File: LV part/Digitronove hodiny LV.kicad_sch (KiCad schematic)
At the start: 92 parts, among them J1 DD4012SB_3V3, J10 Output, J11 Output, J12 Output, J13 -, J14 9V to 170V, J15 Output, J16 Output, J17 Output, J18 Output, J19 Output, J2 +, J20 Output, J21 Output, J22 Output, J24 RCWL-0516, J25 Output, J26 Output, J27 Output, J28 Output, J29 Output, J3 Output, J30 Output, J31 Output, J32 Output, J33 Output, J34 Output, J35 Output, J36 Output, J37 Output, J38 Output, J39 Output, J4 Output, J40 Output, J41 Output, J42 Output, J43 Output, J5 Output, J6 Output, J7 Output, J8 Output, J9 Output, SW1 RESET, SW2 START/STOP, SW3 +1, SW4 SWITCH, U1 74HC595, U2 74HC595, U3 ESP32-WROOM-32, U4 74HC595, U5 74HC595, U6 74HC595, U7 74HC595

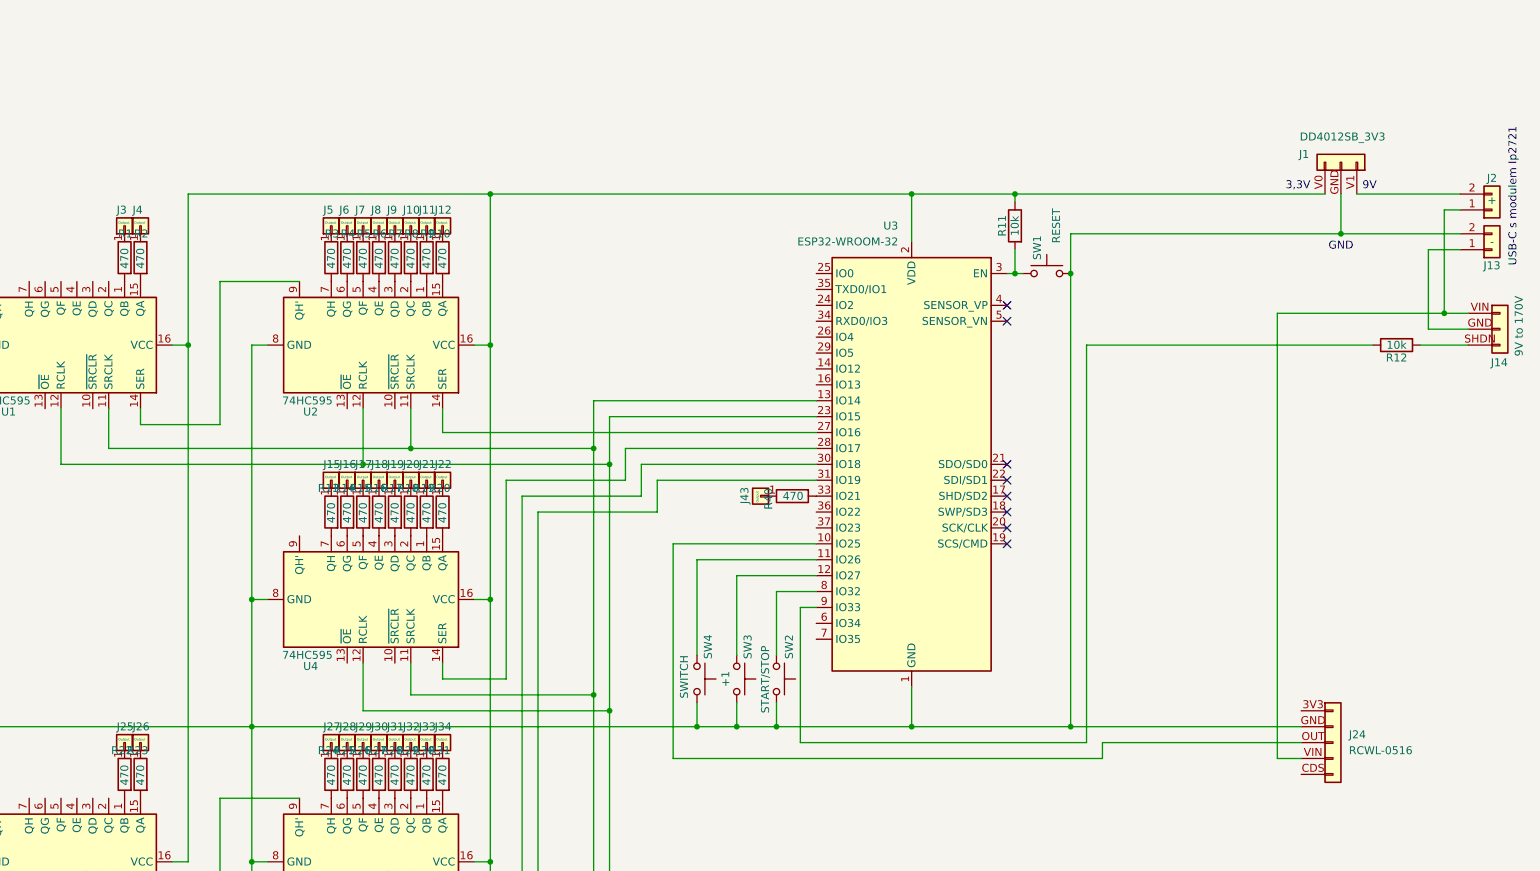
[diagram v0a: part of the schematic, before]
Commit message: LV Schema
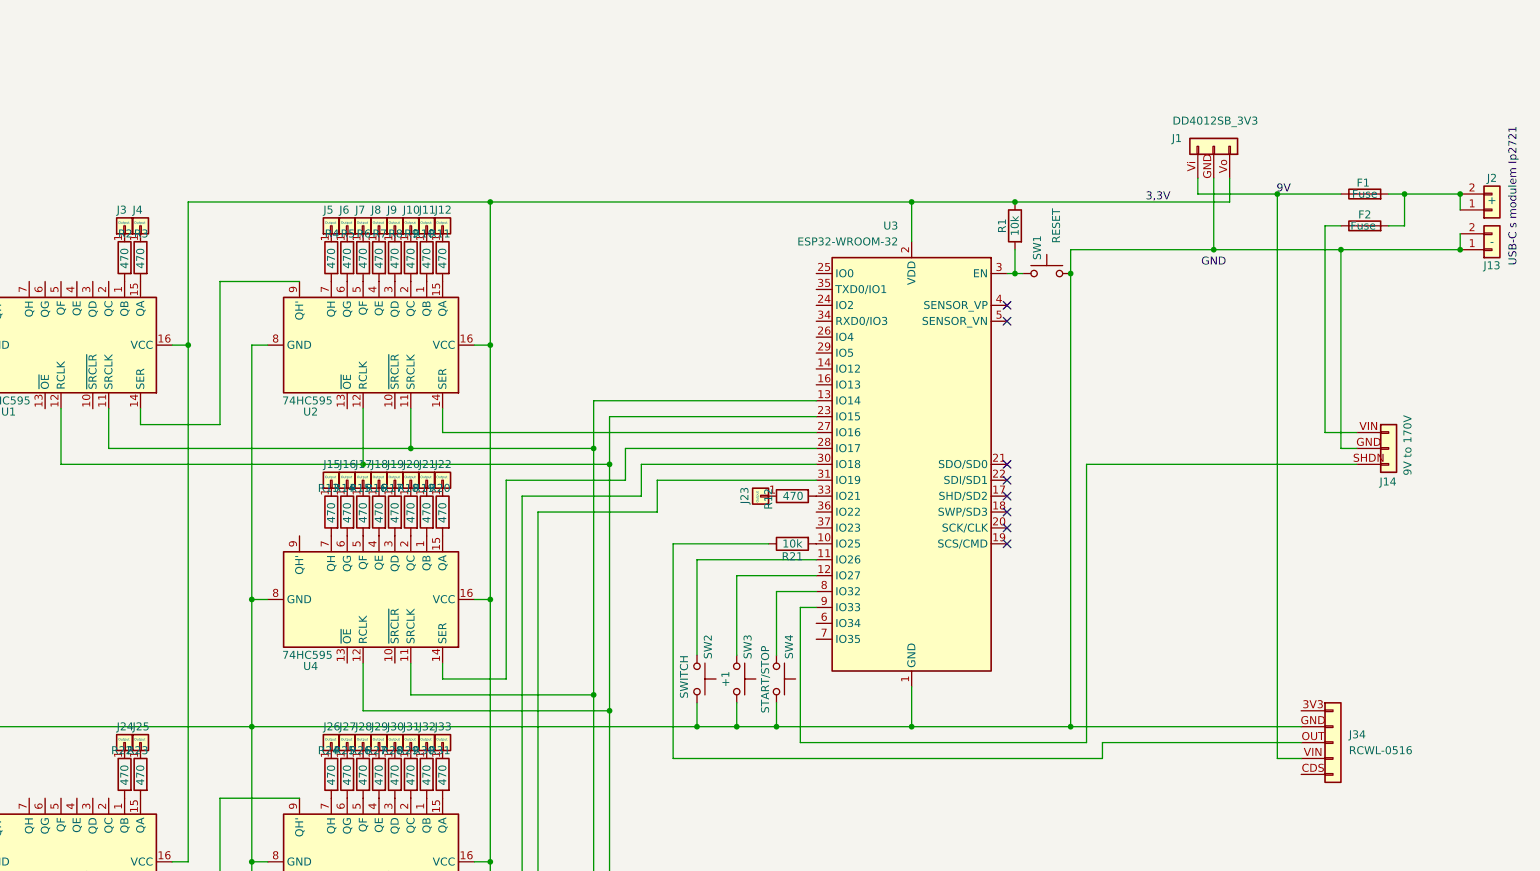
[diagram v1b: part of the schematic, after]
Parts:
- removed J34: Output, symbol Connector_Generic:Conn_01x01
- removed R1: 470, symbol Device:R
- removed R12: 10k, symbol Device:R
- added F1, F2: Fuse, Fuse:Fuse_1812_4532Metric, symbol Device:Fuse
- added J24: Output, Connector_PinHeader_1.00mm:PinHeader_1x01_P1.00mm_Horizontal, symbol Connector_Generic:Conn_01x01
- added R11: 470, Resistor_SMD:R_1206_3216Metric_Pad1.30x1.75mm_HandSolder, symbol Device:R
- added R21: 10k, Resistor_SMD:R_1206_3216Metric_Pad1.30x1.75mm_HandSolder, symbol Device:R
- J1: footprint (none) -> Converter_DCDC:Converter_DCDC_RECOM_R-78HB-0.5L_THT
- J10, J11, J12, J15, J16, J17, J18, J19, J20, J21, J22, J25, J26, J27, J28, J29, J3, J30, J31, J32, J33, J35, J36, J37, J38, J39, J4, J40, J41, J42, J5, J6, J7, J8, J9: footprint (none) -> Connector_PinHeader_1.00mm:PinHeader_1x01_P1.00mm_Horizontal
- J14: footprint (none) -> Connector_PinHeader_1.00mm:PinHeader_1x03_P1.00mm_Horizontal
- J23: renamed from J43; footprint (none) -> Connector_PinHeader_1.00mm:PinHeader_1x01_P1.00mm_Horizontal
- J34: renamed from J24; footprint (none) -> LOGIC-74HC595N_DIP16_:Untitled
- R1: renamed from R11; footprint (none) -> Resistor_SMD:R_1206_3216Metric_Pad1.30x1.75mm_HandSolder
- R10, R13, R14, R15, R16, R17, R18, R19, R2, R20, R22, R23, R24, R25, R26, R27, R28, R29, R3, R30, R31, R32, R33, R34, R35, R36, R37, R38, R39, R4, R5, R6, R7, R8, R9: footprint (none) -> Resistor_SMD:R_1206_3216Metric_Pad1.30x1.75mm_HandSolder
- R12: renamed from R40; footprint (none) -> Resistor_SMD:R_1206_3216Metric_Pad1.30x1.75mm_HandSolder
- SW1, SW3: footprint (none) -> Button_Switch_THT:SW_PUSH_6mm_H4.3mm
- SW2: renamed from SW4; footprint (none) -> Button_Switch_THT:SW_PUSH_6mm_H4.3mm
- SW4: renamed from SW2; footprint (none) -> Button_Switch_THT:SW_PUSH_6mm_H4.3mm
- U1, U2, U4, U5, U6, U7: footprint (none) -> LOGIC-74HC595N_DIP16_:74HC595N
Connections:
- net at J26.1 (Pin_1): now also R24.1; no longer R23.1
- net at J9.1 (Pin_1): now also R8.1; no longer R7.1
- net at U2.3 (QD): now also R8.2; no longer R7.2
- net at R1.1, U1.16 (VCC), U2.16 (VCC)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: now also J1.Vo (Pin_1); no longer J1.V0 (Pin_3)
- net at J1.GND (Pin_2), J13.2 (Pin_2), J34.GND (Pin_2)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: now also J13.1 (Pin_1), J14.GND (Pin_2)
- net at R6.1: now also J7.1 (Pin_1); no longer J8.1 (Pin_1)
- net at R9.1: now also J10.1 (Pin_1); no longer J11.1 (Pin_1)
- net at R22.1: now also J24.1 (Pin_1); no longer J25.1 (Pin_1)
- net at J14.SHDN (Pin_3): now also U3.9 (IO33)
- net at J29.1 (Pin_1): now also R27.1; no longer R26.1
- net at J34.OUT (Pin_3): now also R21.1; no longer U3.10 (IO25)
- net at J12.1 (Pin_1): now also R11.1; no longer R10.1
- net at J32.1 (Pin_1): now also R30.1; no longer R29.1
- net at R31.1: now also J33.1 (Pin_1)
- net at J28.1 (Pin_1): now also R26.1; no longer R25.1
- net at R4.1: now also J5.1 (Pin_1); no longer J6.1 (Pin_1)
- net at J30.1 (Pin_1): now also R28.1; no longer R27.1
- net at J27.1 (Pin_1): now also R25.1; no longer R24.1
- net at U2.2 (QC): now also R9.2; no longer R8.2
- net at J2.2 (Pin_2): now also J2.1 (Pin_1), F1.2, F2.2; no longer J1.V1 (Pin_1)
- net at R5.1: now also J6.1 (Pin_1); no longer J7.1 (Pin_1)
- net at U1.1 (QB): now also R2.2
- net at U1.15 (QA): now also R3.2; no longer R2.2
- net at J3.1 (Pin_1): now also R2.1
- net at J31.1 (Pin_1): now also R29.1; no longer R28.1
- net at R6.2: now also U2.5 (QF); no longer U2.4 (QE)
- net at U2.15 (QA): now also R11.2; no longer R10.2
- net at R3.1: now also J4.1 (Pin_1); no longer J5.1 (Pin_1)
- net at U2.7 (QH): now also R4.2; no longer R3.2
- net at U2.6 (QG): now also R5.2; no longer R4.2
- net at U2.1 (QB): now also R10.2; no longer R9.2
- new net: F2.1, J14.VIN (Pin_1)
- new net: F1.1, J1.Vi (Pin_3), J34.VIN (Pin_4)
- new net: R21.2, U3.10 (IO25)
- new net: J11.1 (Pin_1), R10.1
- new net: J25.1 (Pin_1), R23.1
- new net: J8.1 (Pin_1), R7.1
- new net: R7.2, U2.4 (QE)
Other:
- moved on the sheet: J1, J14
